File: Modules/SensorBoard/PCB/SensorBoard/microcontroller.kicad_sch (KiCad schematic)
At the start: 3 parts, among them J5 PROG, J7 Micro_SD_Card_Det1, U1 ESP32-WROOM-32D

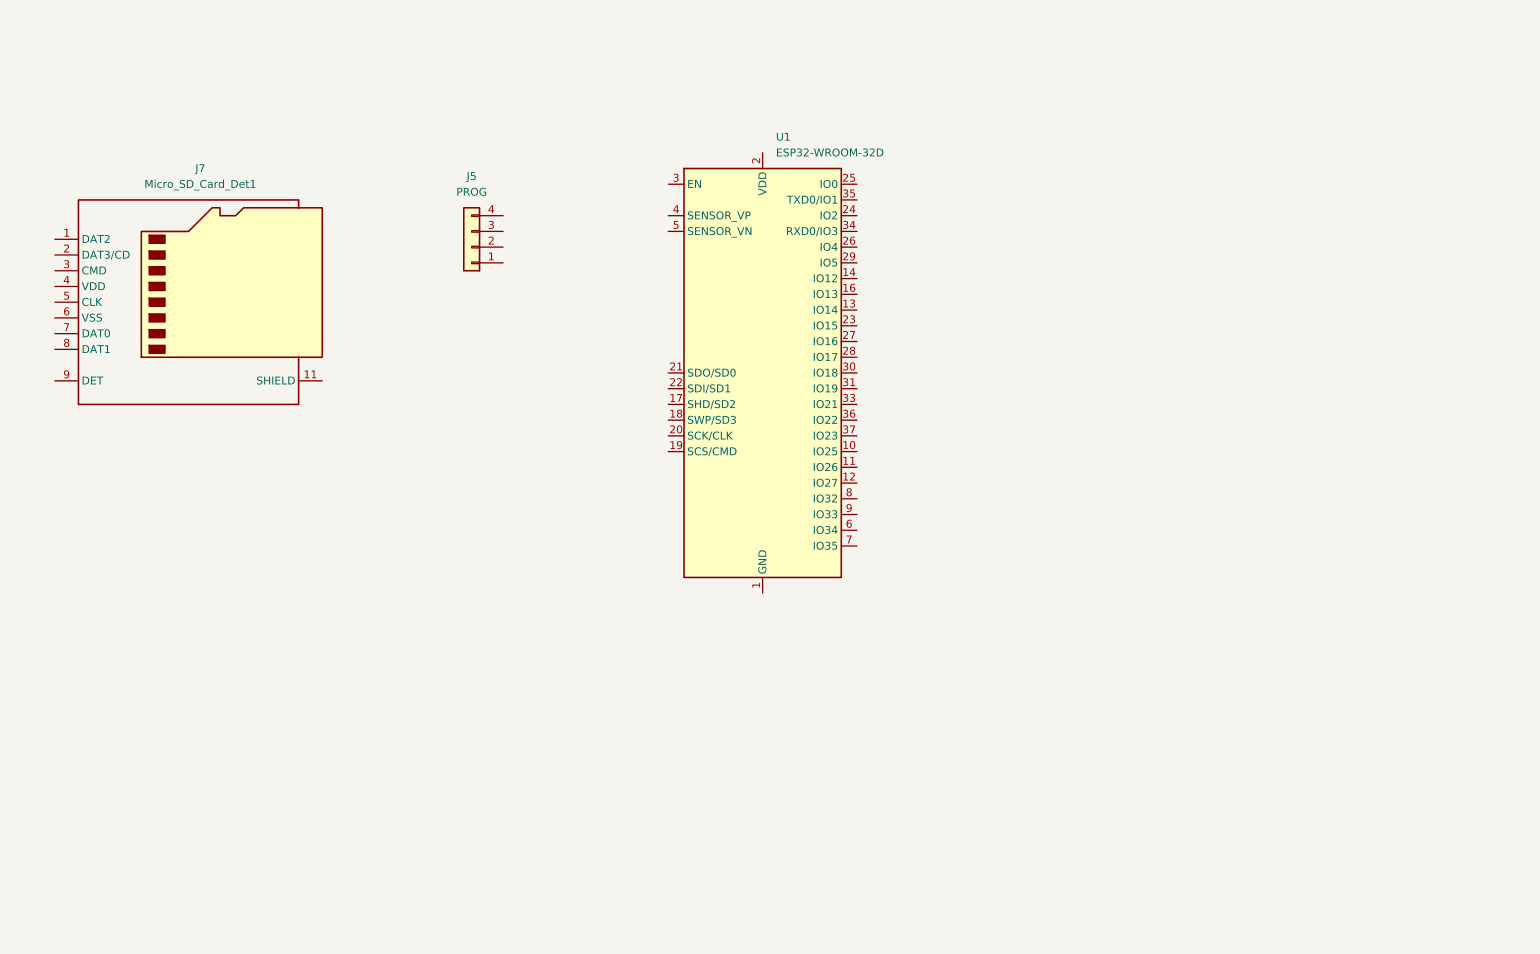
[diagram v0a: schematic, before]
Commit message: Finished Supply board
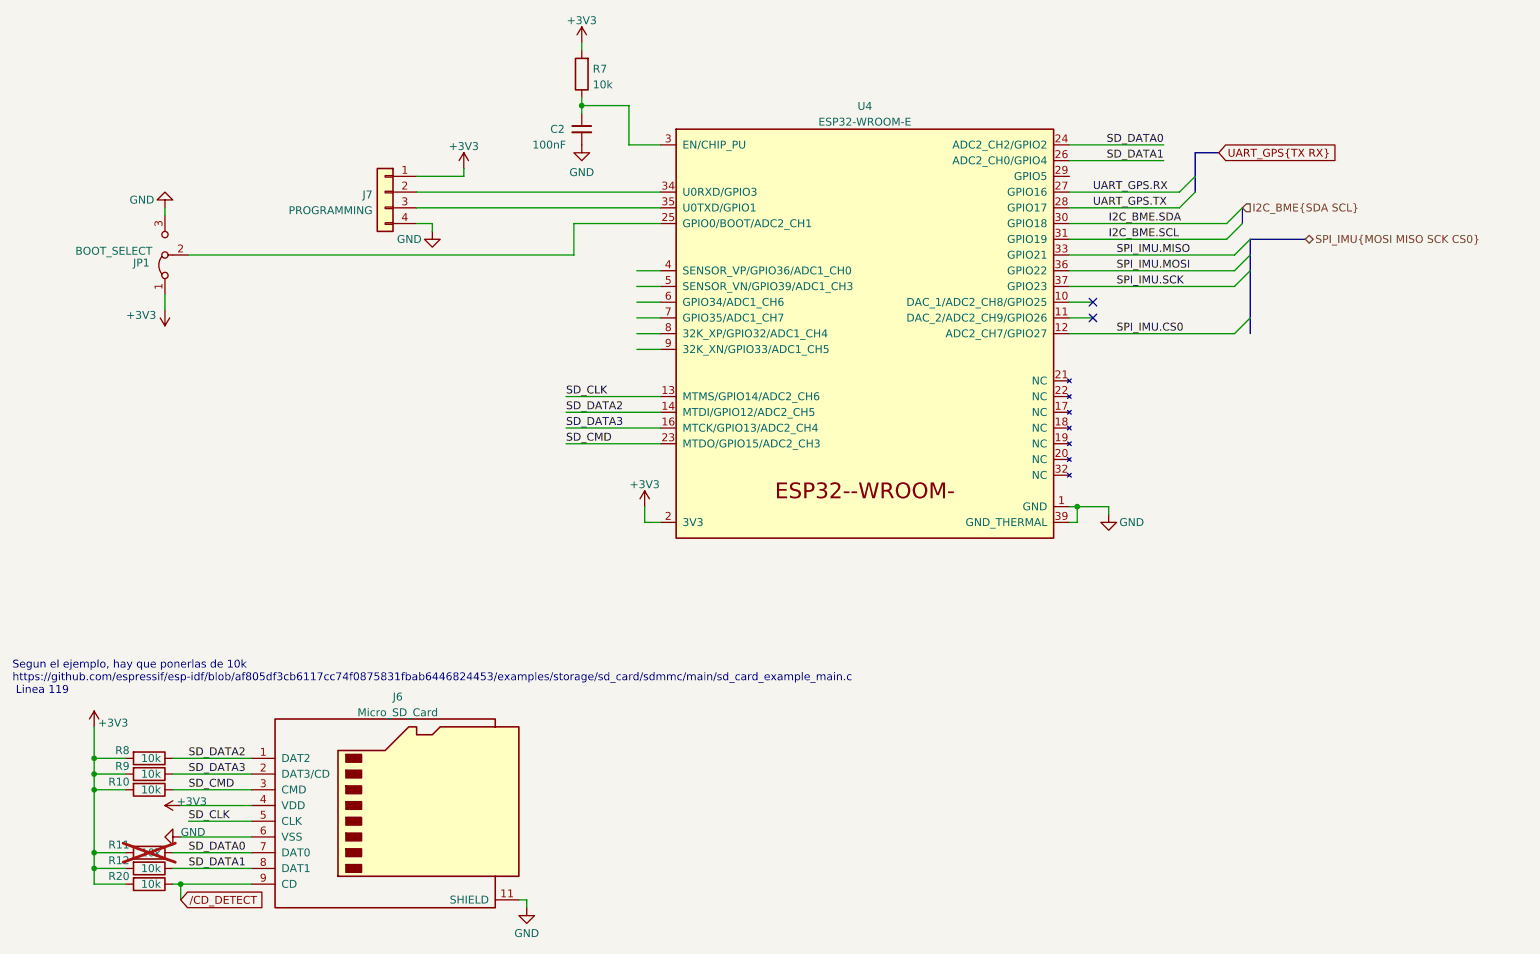
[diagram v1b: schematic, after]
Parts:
- removed J5: PROG, Connector_PinHeader_2.54mm:PinHeader_1x04_P2.54mm_Vertical, symbol Connector_Generic:Conn_01x04
- removed J7: Micro_SD_Card_Det1, IcaroFootprints:microSD-Receptacle-SelfEject, symbol Connector:Micro_SD_Card_Det1
- removed U1: ESP32-WROOM-32D, RF_Module:ESP32-WROOM-32D, symbol RF_Module:ESP32-WROOM-32D
- added C2: 100nF, Capacitor_SMD:C_0603_1608Metric_Pad1.08x0.95mm_HandSolder, symbol Device:C_Small
- added J6: Micro_SD_Card, IcaroFootprints:microSD-Receptacle-SelfEject, symbol Connector:Micro_SD_Card
- added J7: PROGRAMMING, Connector_PinHeader_2.54mm:PinHeader_1x04_P2.54mm_Vertical, symbol Connector_Generic:Conn_01x04
- added JP1: BOOT_SELECT, Connector_PinHeader_2.54mm:PinHeader_1x03_P2.54mm_Vertical, symbol Jumper:Jumper_3_Bridged12
- added R10, R11, R12, R20, R7, R8, R9: 10k, Resistor_SMD:R_0603_1608Metric_Pad0.98x0.95mm_HandSolder, symbol Device:R
- added U4: ESP32-WROOM-E, RF_Module:ESP32-WROOM-32UE, symbol Espressif:ESP32-WROOM-E
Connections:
- new net: C2.1, R7.1, U4.3 (EN/CHIP_PU)
- new net: JP1.2 (C), U4.25 (GPIO0/BOOT/ADC2_CH1)
- new net: J7.2 (Pin_2), U4.34 (U0RXD/GPIO3)
- new net: J7.3 (Pin_3), U4.35 (U0TXD/GPIO1)
- new net +3V3: J6.4 (VDD), J7.1 (Pin_1), JP1.1 (A), R10.2, R11.2, R12.2, R20.2, R7.2, R8.2, R9.2, U4.2 (3V3)
- new net GND: C2.2, J6.11 (SHIELD), J6.6 (VSS), J7.4 (Pin_4), JP1.3 (B), U4.1 (GND), U4.15 (GND), U4.38 (GND), U4.39 (GND_THERMAL)
- new net I2C_BME.SCL: U4.31 (GPIO19)
- new net I2C_BME.SDA: U4.30 (GPIO18)
- new net SD_CLK: J6.5 (CLK), U4.13 (MTMS/GPIO14/ADC2_CH6)
- new net SD_CMD: J6.3 (CMD), R10.1, U4.23 (MTDO/GPIO15/ADC2_CH3)
- new net SD_DATA0: J6.7 (DAT0), R11.1, U4.24 (ADC2_CH2/GPIO2)
- new net SD_DATA1: J6.8 (DAT1), R12.1, U4.26 (ADC2_CH0/GPIO4)
- new net SD_DATA2: J6.1 (DAT2), R8.1, U4.14 (MTDI/GPIO12/ADC2_CH5)
- new net SD_DATA3: J6.2 (DAT3/CD), R9.1, U4.16 (MTCK/GPIO13/ADC2_CH4)
- new net SPI_IMU.CS0: U4.12 (ADC2_CH7/GPIO27)
- new net SPI_IMU.MISO: U4.33 (GPIO21)
- new net SPI_IMU.MOSI: U4.36 (GPIO22)
- new net SPI_IMU.SCK: U4.37 (GPIO23)
- new net UART_GPS.RX: U4.27 (GPIO16)
- new net UART_GPS.TX: U4.28 (GPIO17)
- new net /CD_DETECT: J6.9 (CD), R20.1
- no-connect marks 0 -> 2
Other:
- note added: "Segun el ejemplo, hay que ponerlas de 10k https://github.com/espressif/esp-idf/blob/af805df3cb6117cc74f0875831fbab6446824453/examples/storage/sd_card/sdmmc/main/sd_card_example_main.c Linea 119"
